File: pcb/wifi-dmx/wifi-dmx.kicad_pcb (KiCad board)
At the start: 2 copper layers, 115 x 75 mm, 12 parts, among them J1 Conn_01x16_Socket, J2 Conn_01x16_Socket, J3 USB4110GFA, J5 NC3FAH1, SW1 SW_Push, U1 MAX485E

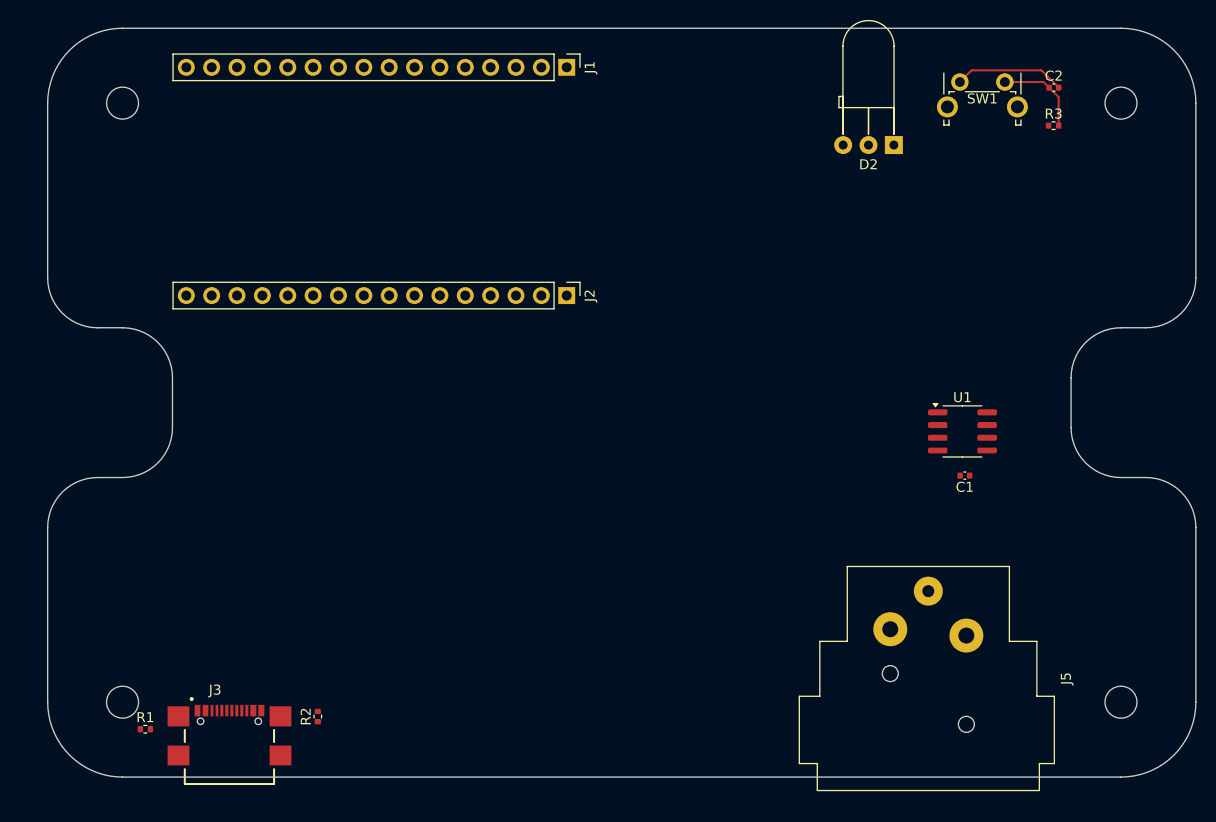
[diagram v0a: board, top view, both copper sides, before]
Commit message: finishing schematic, finishing pcb, integrating pcb-stl with enclosure
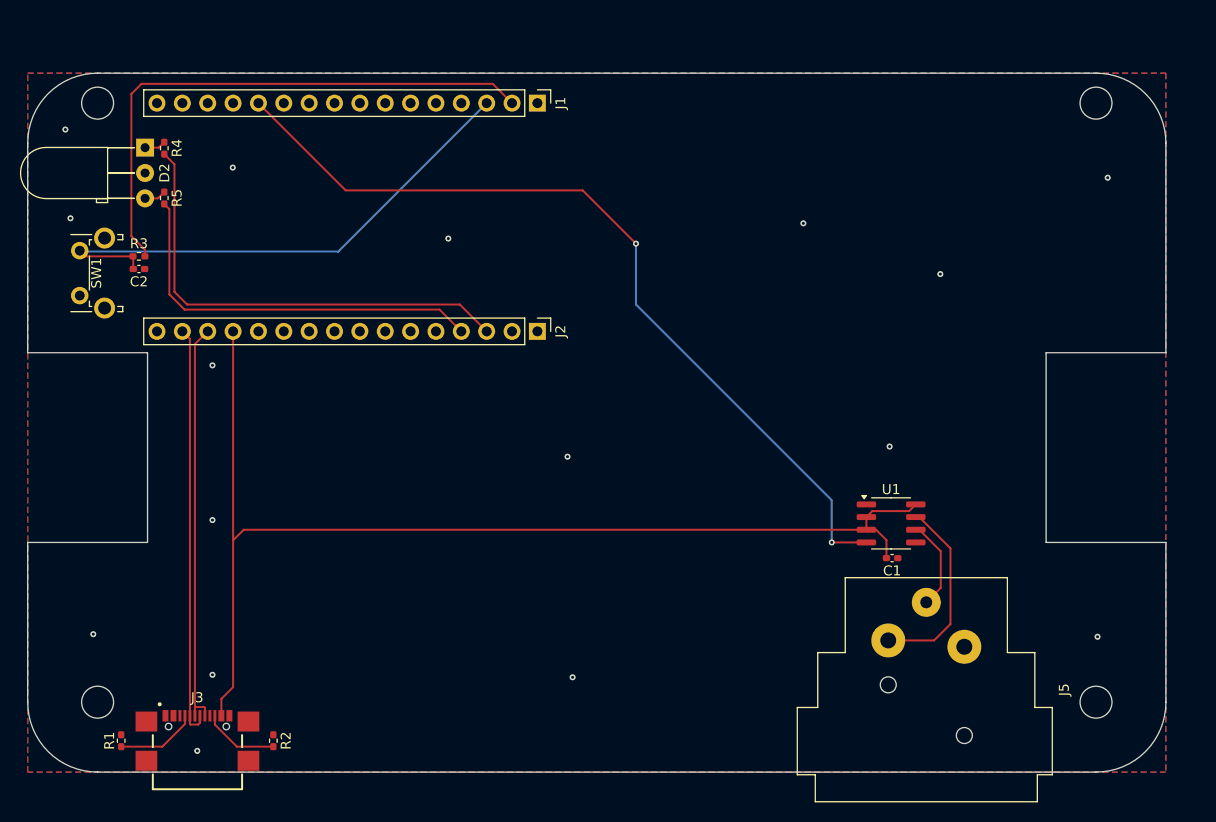
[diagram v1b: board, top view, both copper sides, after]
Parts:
- added R4: 75R, Resistor_SMD:R_0402_1005Metric_Pad0.72x0.64mm_HandSolder, F.Cu at (106.7, 74.5)
- added R5: 75R, Resistor_SMD:R_0402_1005Metric_Pad0.72x0.64mm_HandSolder, F.Cu at (106.7, 79.5)
- C1, C2: footprint Capacitor_SMD:C_0402_1005Metric -> Capacitor_SMD:C_0402_1005Metric_Pad0.74x0.62mm_HandSolder
- R1, R2, R3: footprint Resistor_SMD:R_0402_1005Metric -> Resistor_SMD:R_0402_1005Metric_Pad0.72x0.64mm_HandSolder
- moved C2 93.4 mm to (104.1, 86.6)
- moved R3 92.5 mm to (104.1, 85.3), turned to 180 degrees
- moved SW1 90.7 mm to (98.2, 89.3), turned to 90 degrees
- moved D2 75.0 mm to (104.8, 74.5), turned to -90 degrees
- moved U1 11.7 mm to (179.5, 112.1)
- moved C1 11.0 mm to (179.6, 115.6), turned to 0 degrees
- moved R2 5.07 mm to (117.6, 133.9)
- moved J1 4.63 mm to (144.1, 70.0)
- moved J2 4.63 mm to (144.1, 92.9)
- moved J3 3.25 mm to (110.0, 132.4)
- moved R1 2.68 mm to (102.4, 133.9), turned to 90 degrees
- moved J5 1.14 mm to (186.8, 124.5)
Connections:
- J2 pad 3: LED -> LED_RED
- J2 pad 4: unconnected-(J2-Pin_4-Pad4) -> LED_GREEN
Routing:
- net VCC_5V: track 0.00 -> 113.8 mm
- net TXD1: track 0.00 -> 85.2 mm, vias 0 -> 2
- net VCC_3.3V: track 0.00 -> 56.2 mm
- net LED_RED: track 0.00 -> 47.1 mm
- net BTN_BOOT: track 8.87 -> 53.7 mm
- net D+: track 0.00 -> 41.7 mm
- net D-: track 0.00 -> 41.4 mm
- net LED_GREEN: track 0.00 -> 40.0 mm
- net Net-(U1-B): track 0.00 -> 19.3 mm
- net GND: track 11.1 -> 0.00 mm, vias 0 -> 16
- net Net-(U1-A): track 0.00 -> 9.11 mm
- net Net-(J3-CC1): track 0.00 -> 8.15 mm
- net Net-(J3-CC2): track 0.00 -> 7.66 mm
- net Net-(D2-A2): track 0.00 -> 2.19 mm
- net Net-(D2-A1): track 0.00 -> 2.15 mm
- added copper zone on B.Cu, net GND
- added copper zone on F.Cu, net GND
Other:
- board size 115 x 75 mm -> 114 x 70 mm
